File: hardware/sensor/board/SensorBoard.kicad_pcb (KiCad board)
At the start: 4 copper layers, 40 x 25 mm, 36 parts, among them J1 USB_B_Mini, J2 Conn_01x04_Male, U1 93LC56BT-I/OT, U2 FT232H, U3 74LVC2G17, U4 74LVC1G374, U5 74LVC1G04, Y1 12MHz

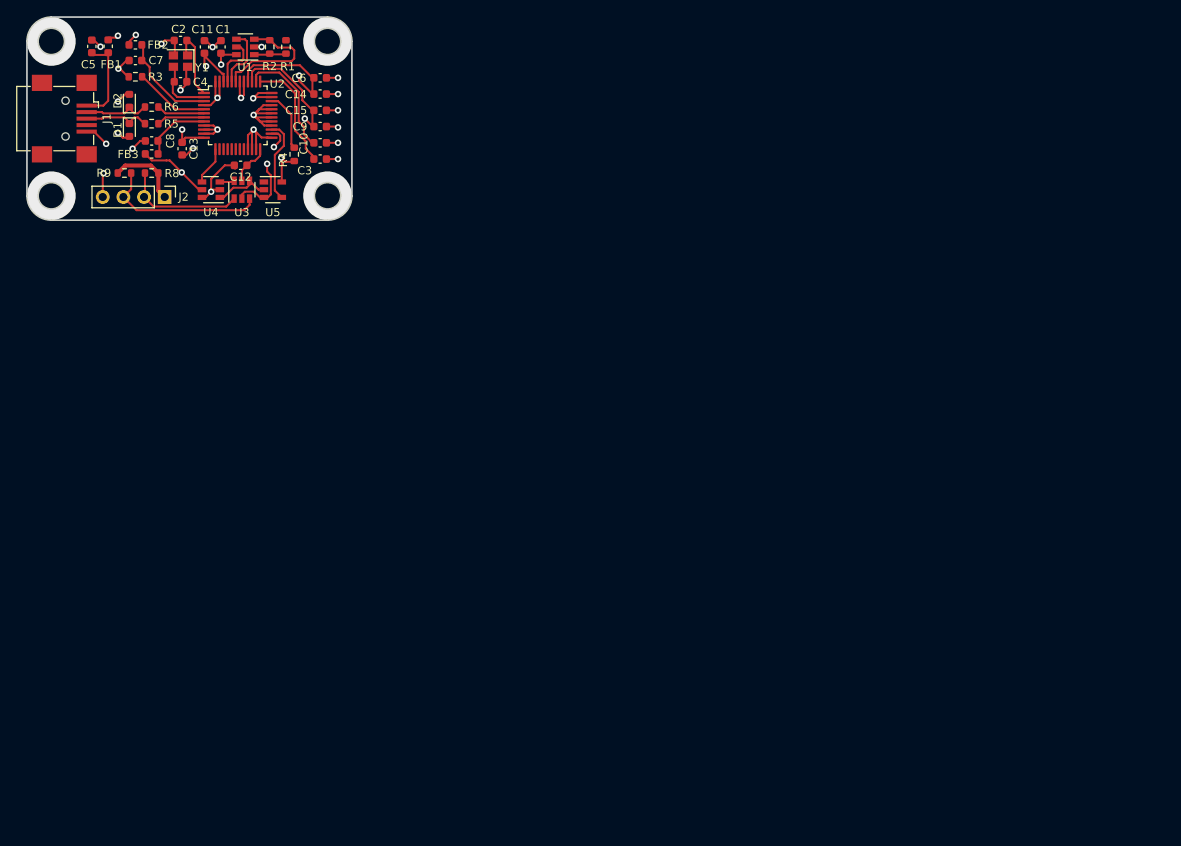
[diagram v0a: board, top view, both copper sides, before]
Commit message: Layout from scratch
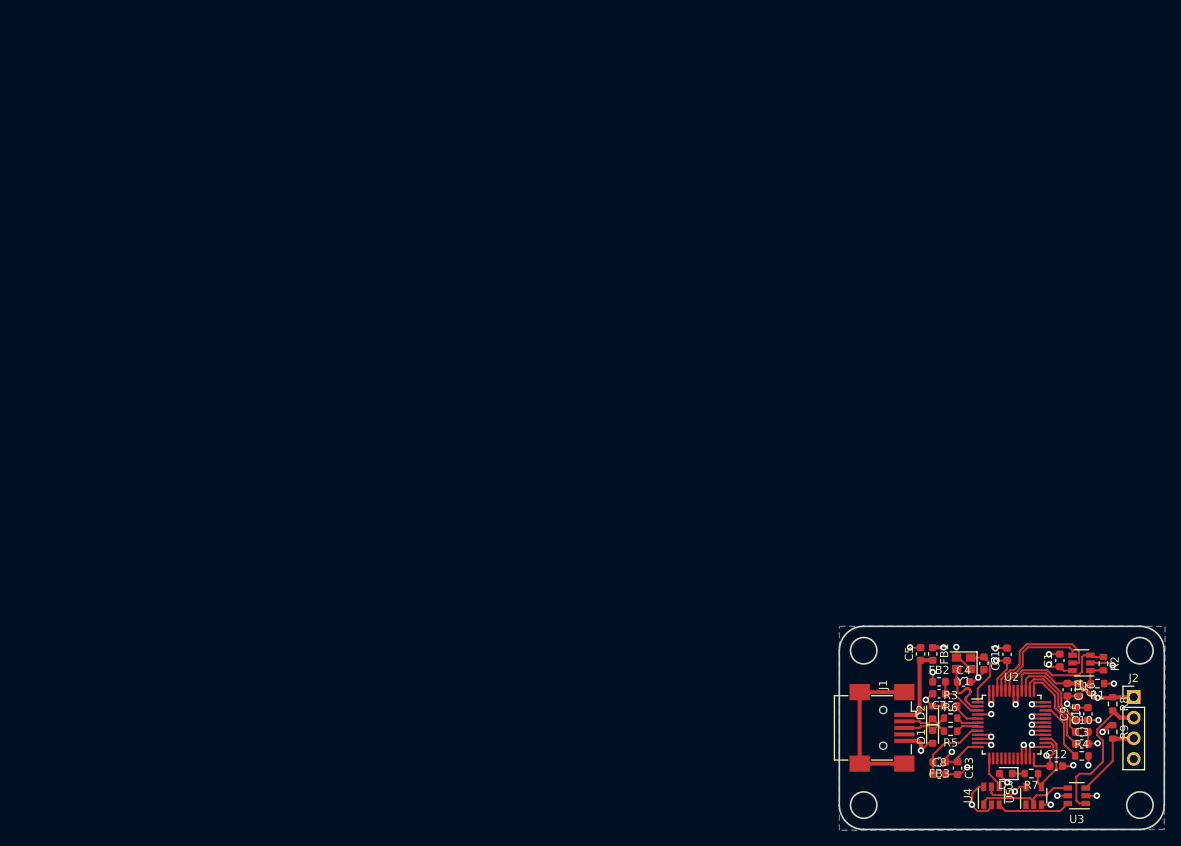
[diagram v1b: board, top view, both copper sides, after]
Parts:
- added D3: LED, LED_SMD:LED_0603_1608Metric, F.Cu at (120.5, 93.1)
- added R7: 1k, Resistor_SMD:R_0603_1608Metric, F.Cu at (123.6, 93.1)
- moved R9 139.8 mm to (133.7, 88.0), turned to 270 degrees
- moved R8 135.1 mm to (133.7, 84.5), turned to 270 degrees
- moved J2 134.2 mm to (136.2, 83.7), turned to 0 degrees
- moved C1 127.9 mm to (127.2, 79.2)
- moved U1 127.8 mm to (129.8, 79.5)
- moved R2 127.7 mm to (132.5, 79.6)
- moved U3 127.0 mm to (129.2, 95.8), turned to 180 degrees
- moved R1 127.0 mm to (131.8, 82.0), turned to 180 degrees
- moved R3 126.8 mm to (113.7, 84.8)
- moved C5 126.5 mm to (110.0, 78.4)
- moved FB2 126.2 mm to (112.3, 81.8)
- moved FB1 126.1 mm to (111.5, 78.4)
- moved C7 125.9 mm to (112.3, 83.3)
- moved J1 125.5 mm to (105.4, 87.5)
- moved C2 125.1 mm to (117.8, 79.5), turned to 270 degrees
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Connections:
- net Net-(C2-Pad1) renamed /CLK+
- net Net-(C3-Pad1) renamed /VCCA
- net Net-(C4-Pad1) renamed /CLK-
- net Net-(J2-Pad2) renamed /Phase1
- net Net-(J2-Pad3) renamed /Phase2
- net Net-(R3-Pad1) renamed /REF
- net Net-(R4-Pad1) renamed /RESET
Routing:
- net Net-(J1-Pad6): track 0.00 -> 19.8 mm
- net GND: track 99.1 -> 79.8 mm, vias 26 -> 27
- net VBUS: track 64.7 -> 46.6 mm, vias 2 -> 3
- net /Phase2: track 20.6 -> 10.1 mm
- net EECS: track 6.52 -> 16.3 mm
- net Net-(U3-Pad6): track 1.82 -> 9.16 mm
- net VCC3V3: track 117.6 -> 111.2 mm, vias 8 -> 10
- net VPHY: track 12.1 -> 6.32 mm
- net /REF: track 9.18 -> 3.38 mm
- net Net-(U3-Pad4): track 7.01 -> 12.8 mm
- net EECLK: track 7.63 -> 13.0 mm
- net /Phase1: track 15.0 -> 18.6 mm
- net VCORE: track 14.4 -> 10.9 mm
- net D+: track 5.88 -> 2.79 mm
- net D-: track 5.88 -> 2.79 mm
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- added copper zone on B.Cu, net GND
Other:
- net class Default: clearance 0.2 -> 0.127
- net class USB removed
- rule trace_clearance: 0.2 -> 0.127
